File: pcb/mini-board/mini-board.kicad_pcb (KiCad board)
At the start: 2 copper layers, 100.3 x 99.7 mm, 44 parts, among them J1 USB_B, J2 EXPBUS1, J3 Serial, J6 UART1, SW1 RESET, SW2 NMI, SW3 SW_SPDT, U1 74AC14, U2 W65C02, U3 CD74HC688, U4 74AC10, U5 SST39SF040, U6 62256-55, U7 CD74HC688, U8 W65C51NxP, U9 MAX232, X1 14 MHz, Y1 1.8432 MHz

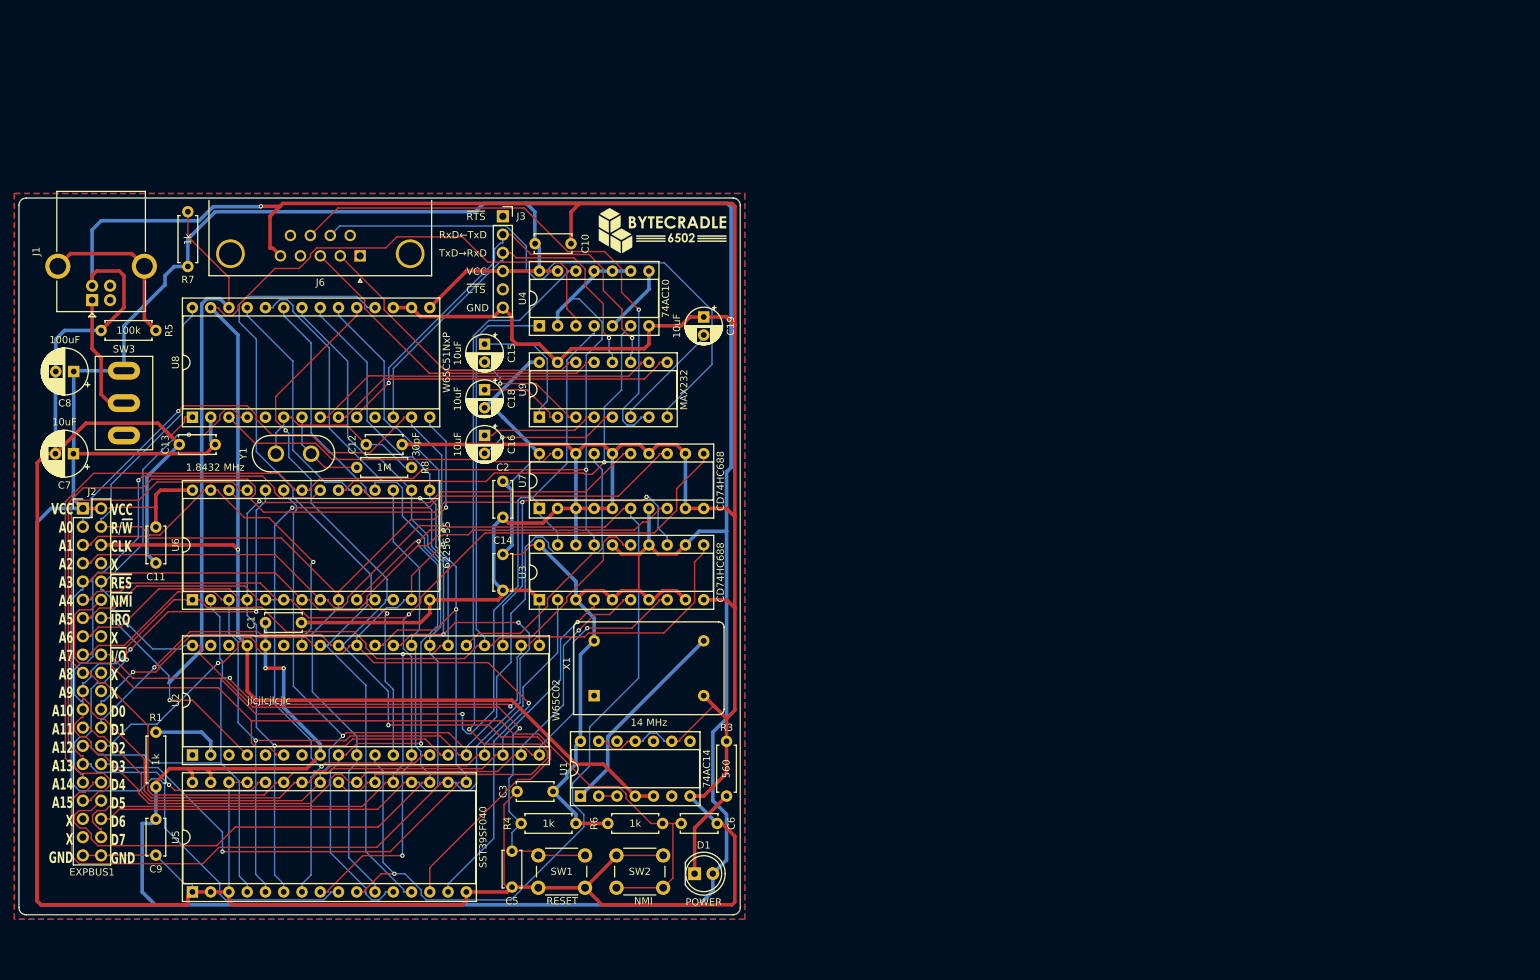
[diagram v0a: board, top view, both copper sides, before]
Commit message: Expanding README.md
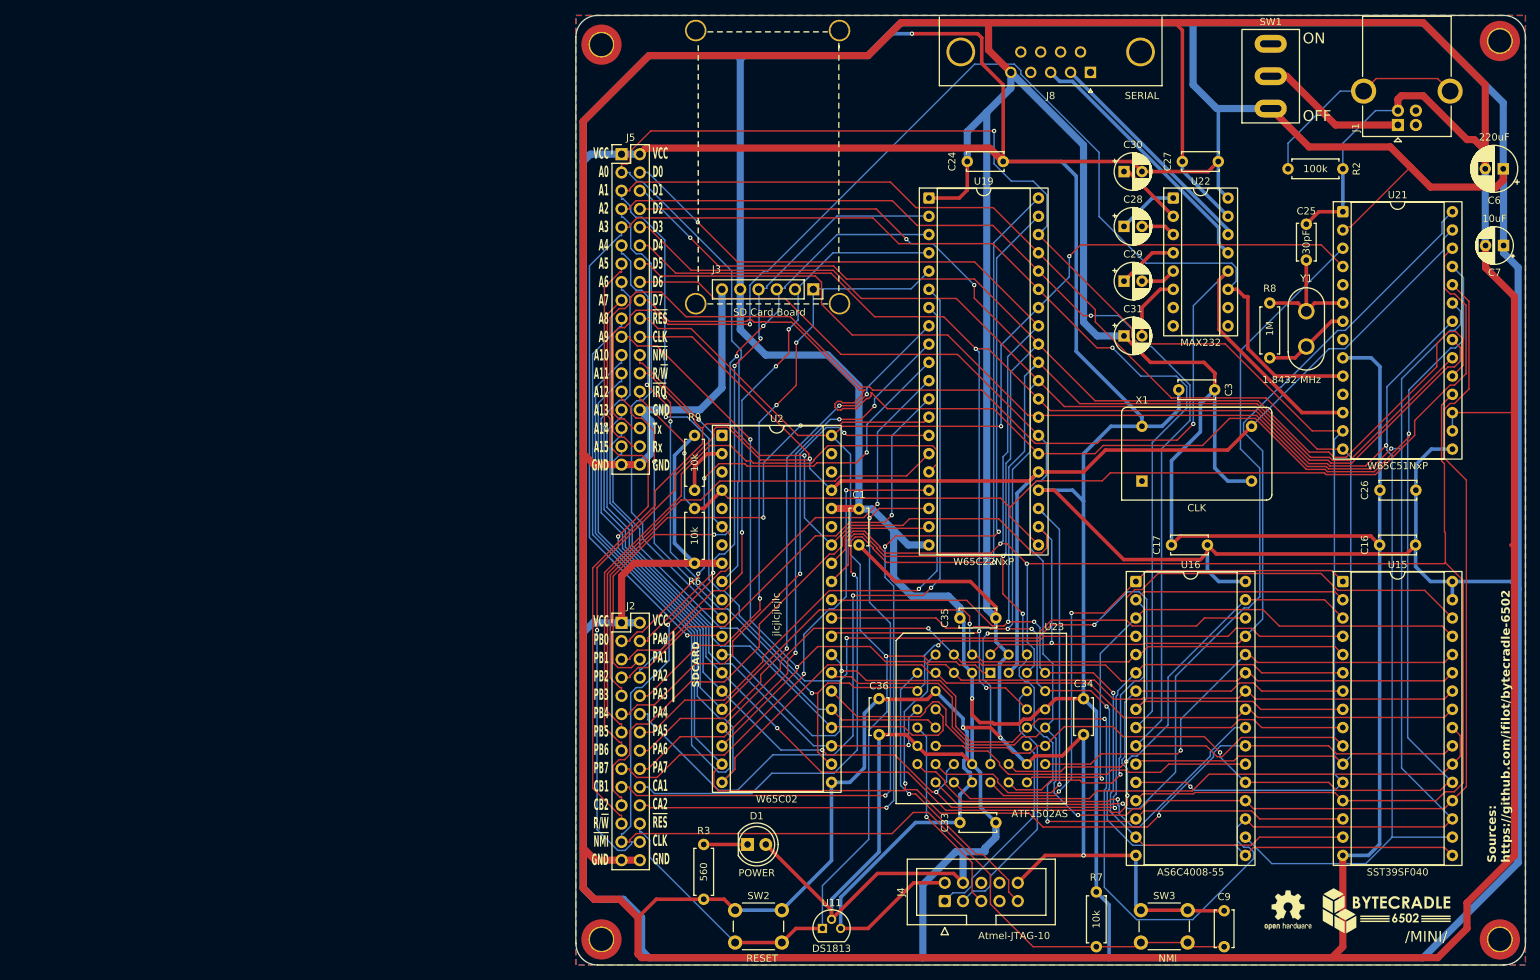
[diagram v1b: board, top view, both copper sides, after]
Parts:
- removed C10, C11, C13, C14, C2, C5: 100nF, Capacitor_THT:C_Disc_D5.0mm_W2.5mm_P5.00mm
- removed C12: 30pF, Capacitor_THT:C_Disc_D5.0mm_W2.5mm_P5.00mm
- removed C15, C18, C19: 10uF, Capacitor_THT:CP_Radial_D5.0mm_P2.50mm
- removed C8: 100uF, Capacitor_THT:CP_Radial_D6.3mm_P2.50mm
- removed J6: UART1, Connector_Dsub:DSUB-9_Male_Horizontal_P2.77x2.84mm_EdgePinOffset4.94mm_Housed_MountingHolesOffset7.48mm
- removed R1, R4: 1k, Resistor_THT:R_Axial_DIN0207_L6.3mm_D2.5mm_P7.62mm_Horizontal
- removed R5: 100k, Resistor_THT:R_Axial_DIN0207_L6.3mm_D2.5mm_P7.62mm_Horizontal
- removed U1: 74AC14, Package_DIP:DIP-14_W7.62mm_Socket
- removed U3, U7: CD74HC688, Package_DIP:DIP-20_W7.62mm_Socket
- removed U4: 74AC10, Package_DIP:DIP-14_W7.62mm_Socket
- removed U5: SST39SF040, Package_DIP:DIP-32_W15.24mm_Socket
- removed U6: 62256-55, Package_DIP:DIP-28_W15.24mm_Socket
- removed U8: W65C51NxP, Package_DIP:DIP-28_W15.24mm_Socket
- removed U9: MAX232, Package_DIP:DIP-16_W7.62mm_Socket
- added C17: 100nF, Capacitor_THT:C_Disc_D5.0mm_W2.5mm_P5.00mm, F.Cu at (214.8, 99.1)
- added C24: 100nF, Capacitor_THT:C_Disc_D5.0mm_W2.5mm_P5.00mm, F.Cu at (186.4, 45.7)
- added C25: 30pF, Capacitor_THT:C_Disc_D5.0mm_W2.5mm_P5.00mm, F.Cu at (228.6, 54.4)
- added C26: 100nF, Capacitor_THT:C_Disc_D5.0mm_W2.5mm_P5.00mm, F.Cu at (243.8, 91.4)
- added C27: 100nF, Capacitor_THT:C_Disc_D5.0mm_W2.5mm_P5.00mm, F.Cu at (216.4, 45.7)
- added C28: 10uF, Capacitor_THT:CP_Radial_D5.0mm_P2.50mm, F.Cu at (203.2, 54.7)
- added C29: 10uF, Capacitor_THT:CP_Radial_D5.0mm_P2.50mm, F.Cu at (203.2, 62.4)
- added C30: 10uF, Capacitor_THT:CP_Radial_D5.0mm_P2.50mm, F.Cu at (203.2, 47.1)
- added C31: 10uF, Capacitor_THT:CP_Radial_D5.0mm_P2.50mm, F.Cu at (203.2, 70.0)
- added C33: 100nF, Capacitor_THT:C_Disc_D5.0mm_W2.5mm_P5.00mm, F.Cu at (185.4, 137.7)
- added C34: 100nF, Capacitor_THT:C_Disc_D5.0mm_W2.5mm_P5.00mm, F.Cu at (197.6, 120.4)
- added C35: 100nF, Capacitor_THT:C_Disc_D5.0mm_W2.5mm_P5.00mm, F.Cu at (180.4, 109.2)
- added C36: 100nF, Capacitor_THT:C_Disc_D5.0mm_W2.5mm_P5.00mm, F.Cu at (169.2, 125.4)
- added G002: OSHW-Logo2_7.3x6mm_SilkScreen, Symbol:OSHW-Logo2_7.3x6mm_SilkScreen, F.Cu at (226.1, 149.9)
- added H1: MountingHole, MountingHole:MountingHole_3.2mm_M3_DIN965_Pad_TopOnly, F.Cu at (130.6, 29.5)
- added H2: MountingHole, MountingHole:MountingHole_3.2mm_M3_DIN965_Pad_TopOnly, F.Cu at (255.5, 29.0)
- added H3: MountingHole, MountingHole:MountingHole_3.2mm_M3_DIN965_Pad_TopOnly, F.Cu at (255.5, 153.9)
- added H4: MountingHole, MountingHole:MountingHole_3.2mm_M3_DIN965_Pad_TopOnly, F.Cu at (130.6, 153.9)
- added J4: Atmel-JTAG-10, Connector_IDC:IDC-Header_2x05_P2.54mm_Vertical, F.Cu at (178.3, 148.6)
- added J5: Conn_02x18_Odd_Even, Connector_PinHeader_2.54mm:PinHeader_2x18_P2.54mm_Vertical, F.Cu at (133.3, 44.7)
- added J8: SERIAL, Connector_Dsub:DSUB-9_Pins_Horizontal_P2.77x2.84mm_EdgePinOffset4.94mm_Housed_MountingHolesOffset4.94mm, F.Cu at (198.6, 33.3)
- added R2: 100k, Resistor_THT:R_Axial_DIN0207_L6.3mm_D2.5mm_P7.62mm_Horizontal, F.Cu at (233.7, 46.7)
- added R9: 10k, Resistor_THT:R_Axial_DIN0207_L6.3mm_D2.5mm_P7.62mm_Horizontal, F.Cu at (143.5, 91.4)
- added U11: DS1813, Package_TO_SOT_THT:TO-92, F.Cu at (161.3, 152.4)
- added U15: SST39SF040, Package_DIP:DIP-32_W15.24mm_Socket, F.Cu at (233.7, 104.1)
- added U16: AS6C4008-55, Package_DIP:DIP-32_W15.24mm_Socket, F.Cu at (204.9, 104.1)
- added U19: W65C22NxP, Package_DIP:DIP-40_W15.24mm_Socket, F.Cu at (176.1, 50.8)
- added U21: W65C51NxP, Package_DIP:DIP-28_W15.24mm_Socket, F.Cu at (233.7, 52.7)
- added U22: MAX232, Package_DIP:DIP-16_W7.62mm_Socket, F.Cu at (210.1, 50.8)
- added U23: ATF1502AS, Package_LCC:PLCC-44_THT-Socket, F.Cu at (184.7, 116.8)
- C16: value 10uF -> 100nF; footprint Capacitor_THT:CP_Radial_D5.0mm_P2.50mm -> Capacitor_THT:C_Disc_D5.0mm_W2.5mm_P5.00mm
- C6: value 100nF -> 220uF; footprint Capacitor_THT:C_Disc_D5.0mm_W2.5mm_P5.00mm -> Capacitor_THT:CP_Radial_D6.3mm_P2.50mm
- C7: footprint Capacitor_THT:CP_Radial_D6.3mm_P2.50mm -> Capacitor_THT:CP_Radial_D5.0mm_P2.50mm
- J2: value EXPBUS1 -> Conn_02x14_Odd_Even; footprint Connector_PinHeader_2.54mm:PinHeader_2x20_P2.54mm_Vertical -> Connector_PinHeader_2.54mm:PinHeader_2x14_P2.54mm_Vertical
- J3: value Serial -> SD Card Board; footprint Connector_PinSocket_2.54mm:PinSocket_1x06_P2.54mm_Vertical -> sdcard-holder:sdcard-socket
- R6, R7: value 1k -> 10k
- SW1: value RESET -> SW_SPDT; footprint Button_Switch_THT:SW_PUSH_6mm -> components:power_switch
- SW2: value NMI -> RESET
- SW3: value SW_SPDT -> NMI; footprint components:power_switch -> Button_Switch_THT:SW_PUSH_6mm
- X1: value 14 MHz -> CLK
- moved C7 201.0 mm to (256.0, 57.4)
- moved J1 183.3 mm to (241.3, 40.6)
- moved R7 162.5 mm to (199.4, 154.9), turned to 90 degrees
- moved SW3 158.1 mm to (205.6, 149.9), turned to 0 degrees
- moved C9 149.6 mm to (217.2, 154.9), turned to 90 degrees
- moved SW1 147.8 mm to (223.6, 33.9), turned to 90 degrees
- moved C6 146.2 mm to (256.0, 46.7), turned to 180 degrees
- moved Y1 139.2 mm to (228.6, 71.5), turned to 90 degrees
- moved G001 138.2 mm to (239.8, 149.9)
- moved C16 130.4 mm to (243.8, 99.1), turned to 180 degrees
- moved R8 121.5 mm to (223.5, 65.4), turned to -90 degrees
- moved C3 103.4 mm to (210.9, 77.5), turned to 0 degrees
- moved U2 86.0 mm to (147.3, 83.8), turned to 0 degrees
- moved C1 84.0 mm to (166.4, 94.1), turned to -90 degrees
- moved X1 81.8 mm to (205.7, 90.2)
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- renumbered G*** to G001
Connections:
- C16 pad 1: Net-(U9-C2+) -> VCC
- C16 pad 2: Net-(U9-C2-) -> GND
- C6 pad 1: ~{NMI} -> VCC
- C9 pad 1: VCC -> ~{NMI}
- J2 pad 10: ~{RES} -> PA3
- J2 pad 11: A4 -> PB4
- J2 pad 12: ~{NMI} -> PA4
- J2 pad 13: A5 -> PB5
- J2 pad 14: ~{IRQC51_1} -> PA5
- J2 pad 15: A6 -> PB6
- J2 pad 16: unconnected-(J2-Pin_16-Pad16) -> PA6
- J2 pad 17: A7 -> PB7
- J2 pad 18: ~{I/O} -> PA7
- J2 pad 19: A8 -> CB1
- J2 pad 20: unconnected-(J2-Pin_20-Pad20) -> CA1
- J2 pad 21: A9 -> CB2
- J2 pad 22: unconnected-(J2-Pin_22-Pad22) -> CA2
- J2 pad 23: A10 -> R/~{W}
- J2 pad 24: D0 -> ~{RES}
- J2 pad 25: A11 -> ~{NMI}
- J2 pad 26: D1 -> CLK
- J2 pad 27: A12 -> GND
- J2 pad 28: D2 -> GND
- J2 pad 3: A0 -> PB0
- J2 pad 4: R/~{W} -> MISO
- J2 pad 5: A1 -> PB1
- J2 pad 6: CLK -> MOSI
- J2 pad 7: A2 -> PB2
- J2 pad 8: unconnected-(J2-Pin_8-Pad8) -> PA2
- J2 pad 9: A3 -> PB3
- J3 pad 1: ~{RTS1} -> PA3
- J3 pad 2: TxD1 -> PA2
- J3 pad 3: RxD1 -> MOSI
- J3 pad 4: VCC -> MISO
- J3 pad 5: ~{CTS1} -> VCC
- R6 pad 1: ~{NMI} -> ~{IRQ}
- R7 pad 1: ~{IRQC51_1} -> ~{NMI}
- SW1 pad 1: GND -> VCC
- SW1 pad 2: ~{RES} -> VIN
- SW2 pad 2: ~{NMI} -> ~{RES}
- SW3 pad 1: VCC -> GND
- SW3 pad 2: VIN -> ~{NMI}
- U2 pad 4: ~{IRQC51_1} -> ~{IRQ}
- X1 pad 8: Net-(X1-OUT) -> CLK
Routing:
- net VCC: track 667.3 -> 1274.0 mm
- net GND: track 766.2 -> 1208.7 mm, vias 1 -> 3
- net D5: track 138.8 -> 334.7 mm, vias 0 -> 3
- net R/~{W}: track 85.1 -> 270.2 mm, vias 1 -> 2
- net D7: track 138.0 -> 312.6 mm
- net ~{IRQ}: track 0.00 -> 165.4 mm, vias 0 -> 1
- net D6: track 134.3 -> 290.5 mm, vias 0 -> 1
- net D0: track 155.8 -> 308.1 mm, vias 1 -> 3
- net D3: track 150.2 -> 287.9 mm, vias 2 -> 3
- net CA1: track 0.00 -> 137.5 mm, vias 0 -> 2
- net A1: track 120.5 -> 255.8 mm, vias 1 -> 2
- net A15: track 202.9 -> 67.7 mm, vias 1 -> 0
- net CA2: track 0.00 -> 134.8 mm, vias 0 -> 3
- net ~{I/O}: track 130.1 -> 0.00 mm, vias 1 -> 0
- net D4: track 175.1 -> 301.0 mm, vias 2 -> 4
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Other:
- board size 100.3 x 99.7 mm -> 132.1 x 132.1 mm
- board text added: "/MINI/"
- board text added: "OFF"
- board text added: "ON"
- board text added: "SDCARD"
- board text added: "Sources: https://github.com/ifilot/bytecradle-6502"
- board text added: "VCC A0 A1 A2 A3 A4 A5 A6 A7 A8 A9 A10 A11 A12 A13 A14 A15 GND"
- board text added: "VCC D0 D1 D2 D3 D4 D5 D6 D7 ~{RES} CLK ~{NMI} R/~{W} ~{IRQ} GND Tx Rx GND"
- board text added: "VCC PA0 PA1 PA2 PA3 PA4 PA5 PA6 PA7 CA1 CA2 ~{RES} CLK GND"
- board text added: "VCC PB0 PB1 PB2 PB3 PB4 PB5 PB6 PB7 CB1 CB2 R/~{W} ~{NMI} GND"
- board text removed: "GND"
- board text removed: "RxD←TxD"
- board text removed: "TxD→RxD"
- board text removed: "VCC"
- board text removed: "VCC A0 A1 A2 A3 A4 A5 A6 A7 A8 A9 A10 A11 A12 A13 A14 A15 X X GND"
- board text removed: "VCC R/~{W} CLK X ~{RES} ~{NMI} ~{IRQ} X ~{I/O} X X D0 D1 D2 D3 D4 D5 D6 D7 GND"
- board text removed: "~{CTS}"
- board text removed: "~{RTS}"
